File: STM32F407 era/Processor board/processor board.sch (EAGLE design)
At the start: 33 parts, among them IC1 REG1117, Q1 25 MHz, U2 MAX13052ESA+, X1 MINI-USB-SCHIELD-32005-201, X2 057-010-1

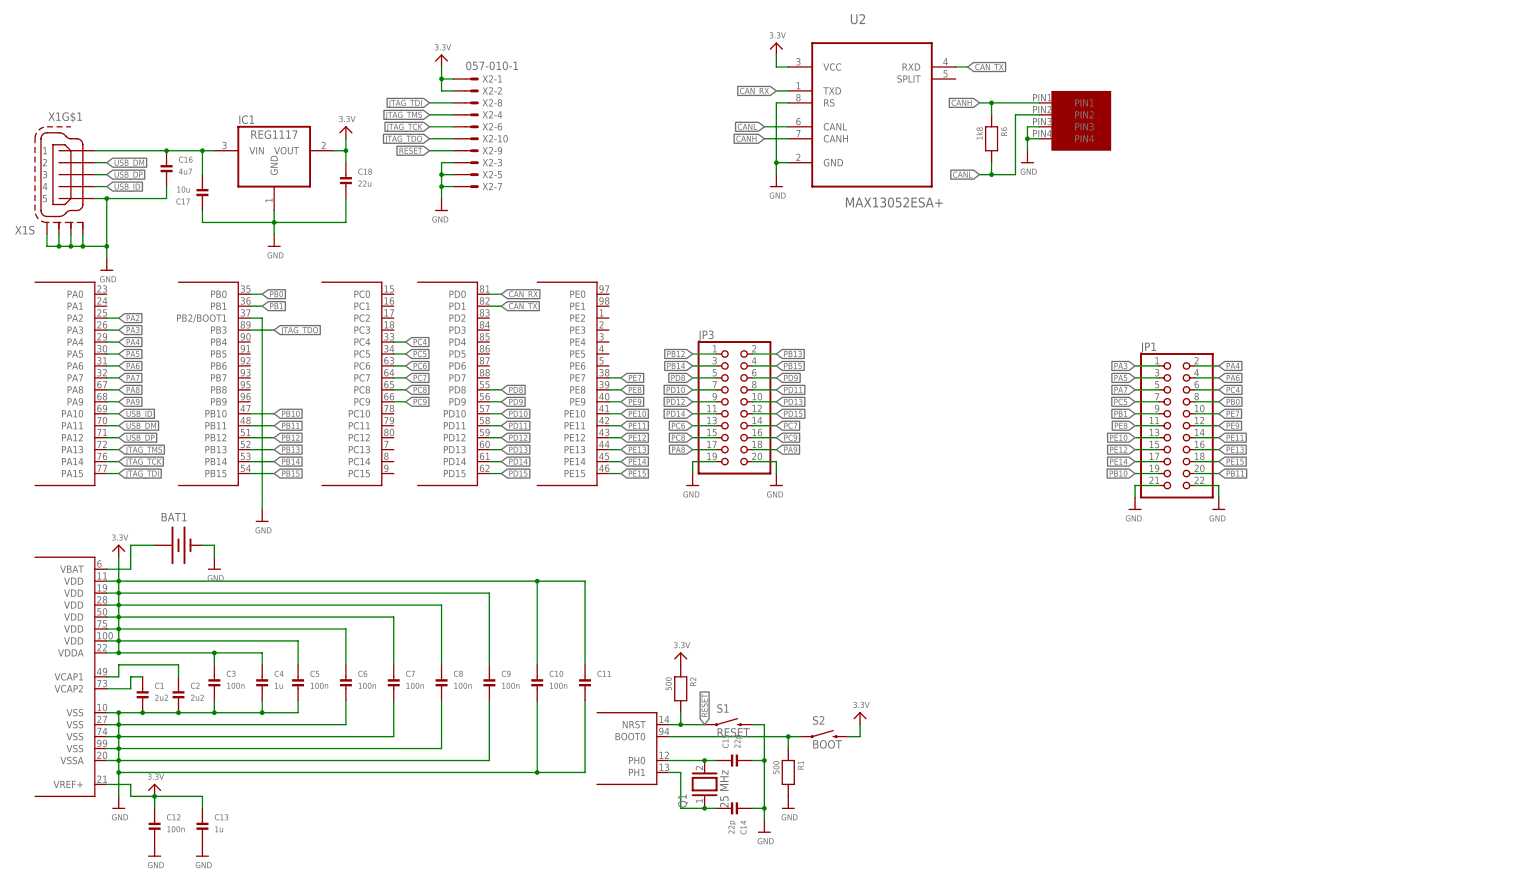
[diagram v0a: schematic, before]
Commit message: finished v 0.1 of processor board layout
TA DAAAAAA!
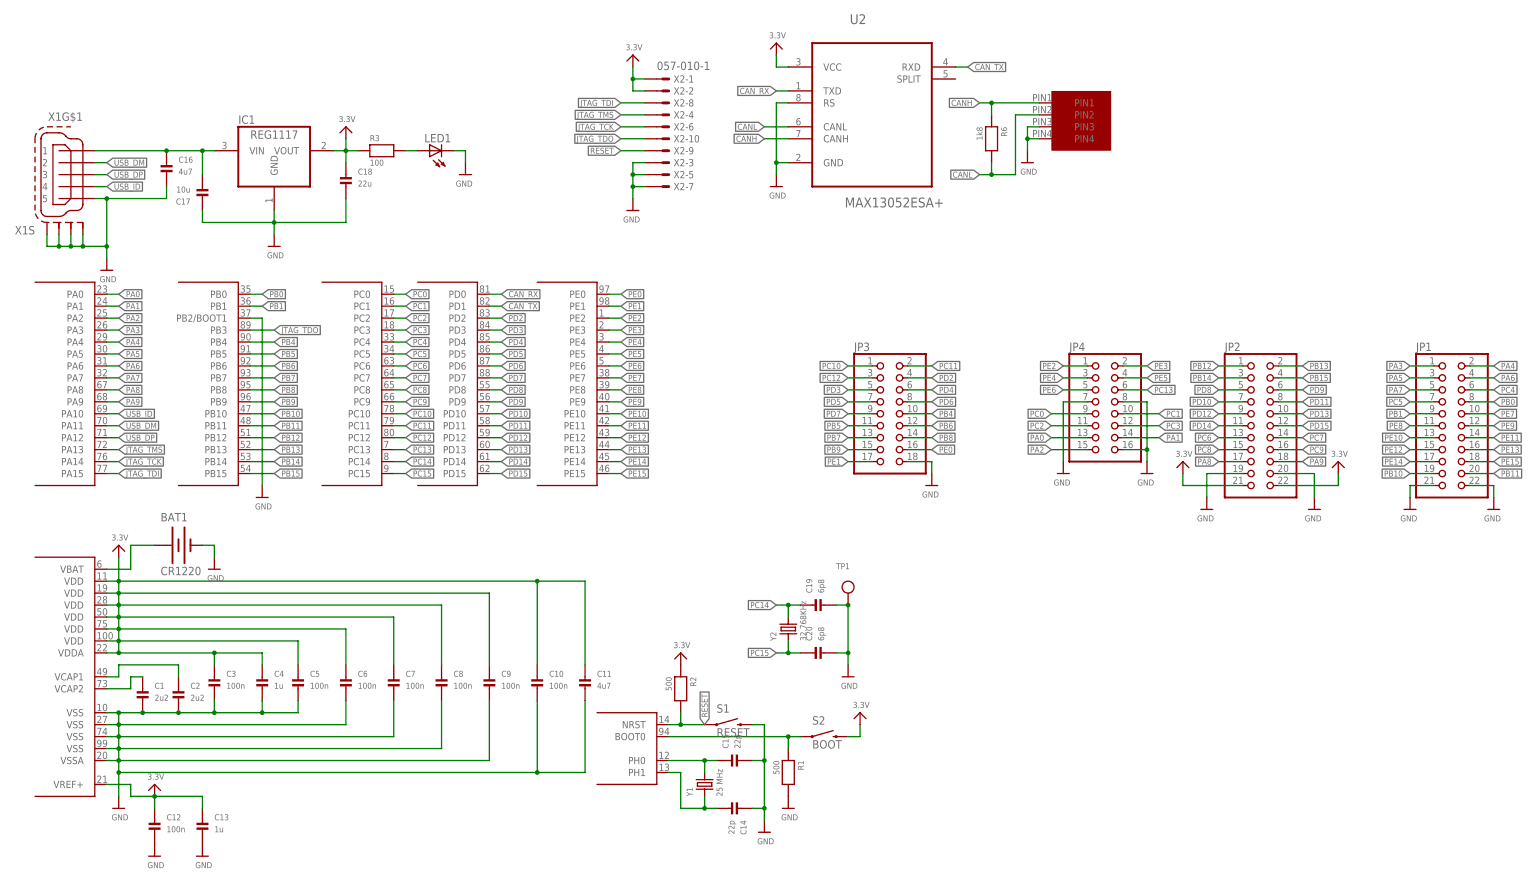
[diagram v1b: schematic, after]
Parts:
- removed Q1: 25 MHz, special:XTAL/S
- added C19, C20: 6p8, microbuilder:CAP_CERAMIC_0402MP
- added JP2: (no value), pinhead:PINHD-2X11
- added JP4: (no value), pinhead:PINHD-2X8
- added LED1: (no value), led:LEDCHIPLED_1206
- added R3: 100, microbuilder:RESISTOR_0402MP
- added TP1: (no value), microbuilder:TESTPOINT0.1"
- added Y1: 25 MHz, microbuilder:CRYSTAL2.5X2.0MM
- added Y2: 32.768KHz, microbuilder:CRYSTAL32.768
- BAT1: value (none) -> CR1220
- C11: value (none) -> 4u7
- JP3: device pinhead:PINHD-2X10 -> pinhead:PINHD-2X9
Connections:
- new net N$5: LED1.A, R3.2
- new net PA0: JP4.13, U1G$2.PA0
- new net PA1: JP4.14, U1G$2.PA1
- new net PB4: JP3.10, U1G$3.PB4
- new net PB5: JP3.11, U1G$3.PB5
- new net PB6: JP3.12, U1G$3.PB6
- new net PB7: JP3.13, U1G$3.PB7
- new net PB8: JP3.14, U1G$3.PB8
- new net PB9: JP3.15, U1G$3.PB9
- new net PC0: JP4.9, U1G$4.PC0
- new net PC1: JP4.10, U1G$4.PC1
- new net PC10: JP3.1, U1G$4.PC10
- new net PC11: JP3.2, U1G$4.PC11
- new net PC12: JP3.3, U1G$4.PC12
- new net PC13: JP4.6, U1G$4.PC13
- new net PC14: C19.P$1, U1G$4.PC14, Y2.2
- new net PC15: C20.P$1, U1G$4.PC15, Y2.1
- new net PC2: JP4.11, U1G$4.PC2
- new net PC3: JP4.12, U1G$4.PC3
- new net PD2: JP3.4, U1G$5.PD2
- new net PD3: JP3.5, U1G$5.PD3
- new net PD4: JP3.6, U1G$5.PD4
- new net PD5: JP3.7, U1G$5.PD5
- new net PD6: JP3.8, U1G$5.PD6
- new net PD7: JP3.9, U1G$5.PD7
- new net PE0: JP3.16, U1G$6.PE0
- new net PE1: JP3.17, U1G$6.PE1
- new net PE2: JP4.1, U1G$6.PE2
- new net PE3: JP4.2, U1G$6.PE3
- new net PE4: JP4.3, U1G$6.PE4
- new net PE5: JP4.4, U1G$6.PE5
- new net PE6: JP4.5, U1G$6.PE6
- net 3.3V: now also JP2.21, JP2.22, R3.1
- net GND: now also C19.P$2, C20.P$2, JP2.19, JP2.20, JP3.18, JP4.16, JP4.7, JP4.8, LED1.C, TP1.P$1; no longer JP3.19, JP3.20
- net N$1: now also Y1.2; no longer Q1.2
- net N$11: now also Y1.1; no longer Q1.1
- net PA2: now also JP4.15
- net PA8: now also JP2.17; no longer JP3.17
- net PA9: now also JP2.18; no longer JP3.18
- net PB12: now also JP2.1; no longer JP3.1
- net PB13: now also JP2.2; no longer JP3.2
- net PB14: now also JP2.3; no longer JP3.3
- net PB15: now also JP2.4; no longer JP3.4
- net PC6: now also JP2.13; no longer JP3.13
- net PC7: now also JP2.14; no longer JP3.14
- net PC8: now also JP2.15; no longer JP3.15
- net PC9: now also JP2.16; no longer JP3.16
- net PD10: now also JP2.7; no longer JP3.7
- net PD11: now also JP2.8; no longer JP3.8
- net PD12: now also JP2.9; no longer JP3.9
- net PD13: now also JP2.10; no longer JP3.10
- net PD14: now also JP2.11; no longer JP3.11
- net PD15: now also JP2.12; no longer JP3.12
- net PD8: now also JP2.5; no longer JP3.5
- net PD9: now also JP2.6; no longer JP3.6
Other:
- moved on the sheet: JP1, X2-1, X2-10, X2-2, X2-3, X2-4, X2-5, X2-6, X2-7, X2-8, X2-9
